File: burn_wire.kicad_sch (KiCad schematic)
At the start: 13 parts, among them J2 Conn_01x01_Pin, J3 Conn_01x01_Pin, Q5 NMOS, U5 74LVC1G08

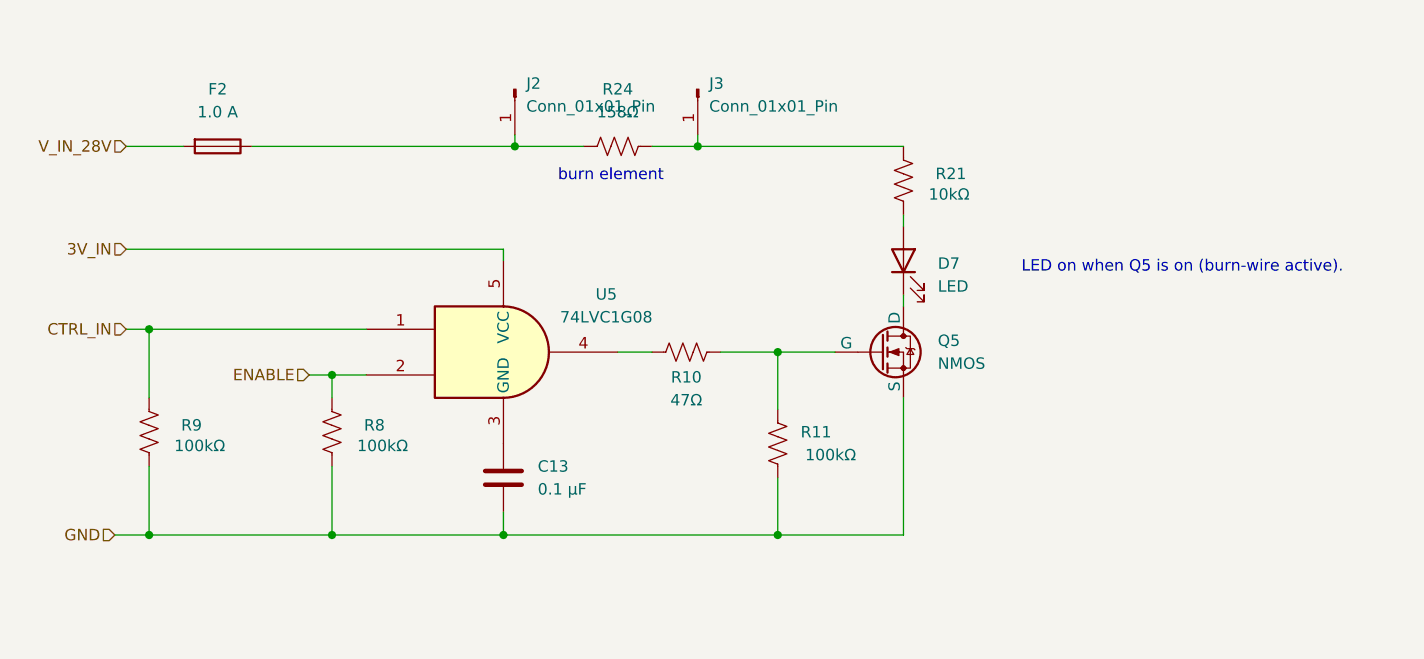
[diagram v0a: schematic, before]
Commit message: Made changes to schematic
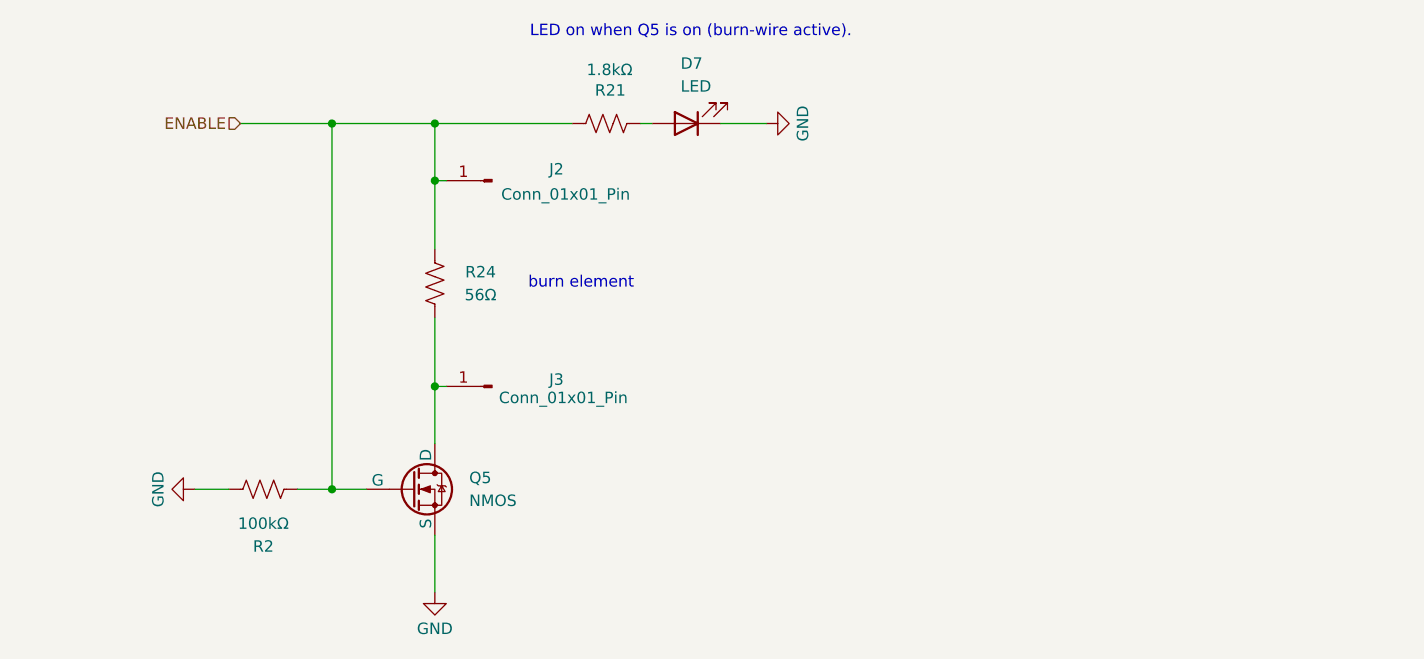
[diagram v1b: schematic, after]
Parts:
- removed C13: 0.1 µF, Capacitor_SMD:C_0603_1608Metric, symbol Device:C
- removed F2: 1.0 A, Fuse:Fuse_1812_4532Metric, symbol Device:Fuse
- removed R10: 47Ω, Resistor_SMD:R_0201_0603Metric, symbol Device:R_US
- removed R11, R8, R9: 100kΩ, Resistor_SMD:R_0201_0603Metric, symbol Device:R_US
- removed U5: 74LVC1G08, Package_TO_SOT_SMD:SOT-23-5, symbol 74xGxx:74LVC1G08
- added R2: 100kΩ, Resistor_SMD:R_0201_0603Metric, symbol Device:R_US
- R21: value 10kΩ -> 1.8kΩ
- R24: value 158Ω -> 56Ω
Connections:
- net ENABLE: now also J2.1 (Pin_1), Q5.2 (G), R21.1, R24.2, R2.2
- net GND: now also D7.1 (K), R2.1
- net at J3.1 (Pin_1), R24.1: now also Q5.1 (D); no longer R21.1
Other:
- moved on the sheet: D7, J2, J3, Q5, R21, R24
